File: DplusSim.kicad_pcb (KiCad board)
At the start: 2 copper layers, 40 x 60 mm, 19 parts, among them J10 K15 -, J11 Summer +, J3 Summer -, J7 Landstr. +, J8 Landstr. -, J9 K15 +, Q2 IRF7404, U5 LTV-847

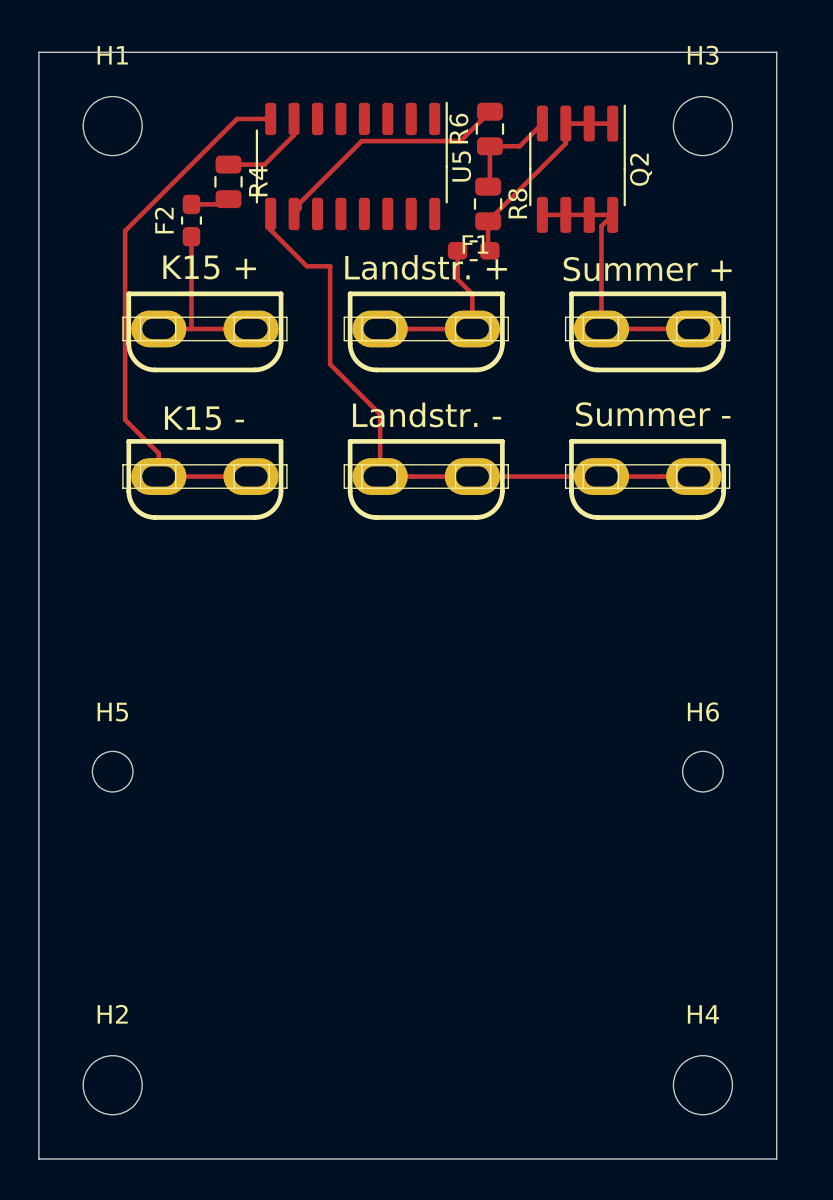
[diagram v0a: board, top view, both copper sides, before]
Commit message: x
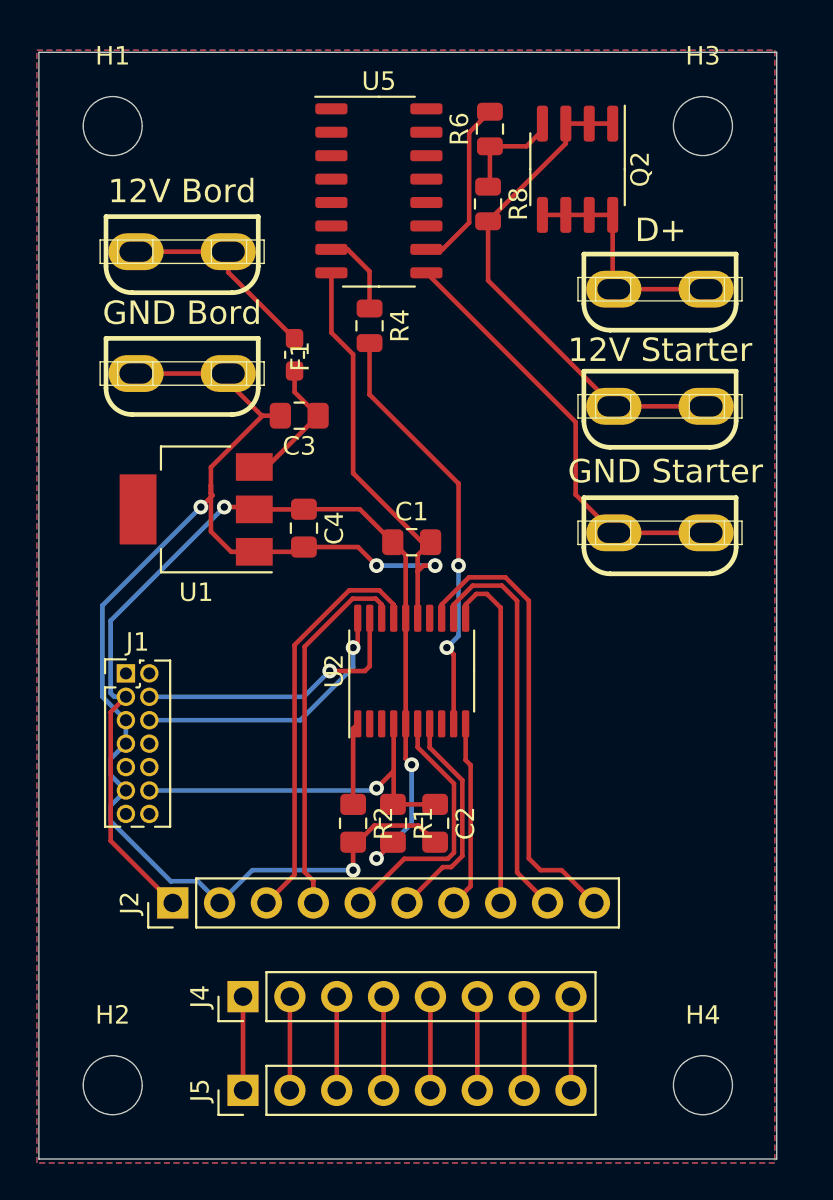
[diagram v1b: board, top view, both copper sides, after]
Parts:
- removed F2: Polyfuse, Resistor_SMD:R_0603_1608Metric_Pad1.05x0.95mm_HandSolder
- removed H5, H6: MountingHole, MountingHole:MountingHole_2.2mm_M2
- removed J10: K15 -, MyComponents:FASTON-6_3mm
- removed J9: K15 +, MyComponents:FASTON-6_3mm
- added C1: 100n, Capacitor_SMD:C_0805_2012Metric_Pad1.15x1.40mm_HandSolder, F.Cu at (29.2, 35.6)
- added C2: C, Capacitor_SMD:C_0805_2012Metric_Pad1.15x1.40mm_HandSolder, F.Cu at (30.5, 50.8)
- added C3: C, Capacitor_SMD:C_0805_2012Metric_Pad1.15x1.40mm_HandSolder, F.Cu at (23.1, 28.7)
- added C4: C, Capacitor_SMD:C_0805_2012Metric_Pad1.15x1.40mm_HandSolder, F.Cu at (23.4, 34.8)
- added J1: Conn_02x07_Odd_Even, Connector_PinHeader_1.27mm:PinHeader_2x07_P1.27mm_Vertical, F.Cu at (13.7, 42.7)
- added J2: Conn_01x10, Connector_PinHeader_2.54mm:PinHeader_1x10_P2.54mm_Vertical, F.Cu at (16.3, 55.1)
- added J4: Conn_01x08, Connector_PinHeader_2.54mm:PinHeader_1x08_P2.54mm_Vertical, F.Cu at (20.1, 60.2)
- added J5: Conn_01x08, Connector_PinHeader_2.54mm:PinHeader_1x08_P2.54mm_Vertical, F.Cu at (20.1, 65.3)
- added J6: 12V Starter, MyComponents:FASTON-6_3mm, F.Cu at (42.7, 28.2)
- added R1: R, Resistor_SMD:R_0805_2012Metric_Pad1.15x1.40mm_HandSolder, F.Cu at (28.2, 50.8)
- added R2: R, Resistor_SMD:R_0805_2012Metric_Pad1.15x1.40mm_HandSolder, F.Cu at (26.0, 50.8)
- added U1: LT1117-3.3, Package_TO_SOT_SMD:SOT-223, F.Cu at (17.5, 33.8)
- added U2: STM32L031F4Px, Package_SO:TSSOP-20_4.4x6.5mm_P0.65mm, F.Cu at (29.2, 42.5)
- J11: value Summer + -> D+
- J3: value Summer - -> GND Starter
- J7: value Landstr. + -> 12V Bord
- J8: value Landstr. - -> GND Bord
- moved J8 14.4 mm to (16.8, 26.4)
- moved J7 13.9 mm to (16.8, 19.8)
- moved F1 11.2 mm to (22.9, 25.4), turned to 90 degrees
- moved R4 10.9 mm to (26.9, 23.8)
- moved J3 3.13 mm to (42.7, 35.1)
- moved J11 2.26 mm to (42.7, 21.8)
- moved U5 1.65 mm to (27.4, 14.0), turned to 0 degrees
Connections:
- net /Warn_plus renamed /Dplus
- J3 pad 1: GND -> GNDA
- Q2 pad 1: +12V -> +12VA
- Q2 pad 2: +12V -> +12VA
- Q2 pad 3: +12V -> +12VA
- R4 pad 2: /K15_plus -> /Dplus_out
- R8 pad 2: +12V -> +12VA
- U5 pad 8: /K15_minus -> GND
- U5 pad 9: GND -> GNDA
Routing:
- net GND: track 34.4 -> 96.9 mm, vias 0 -> 4
- net +3V3: track 0.00 -> 56.0 mm, vias 0 -> 3
- net /K15_minus: track 29.5 -> 0.00 mm
- net +12VA: track 0.00 -> 27.4 mm
- net /SPI_MOSI: track 0.00 -> 25.1 mm
- net GNDA: track 0.00 -> 23.3 mm
- net /Dplus_out: track 0.00 -> 23.1 mm, vias 0 -> 2
- net /I2C_SCL: track 0.00 -> 22.3 mm
- net /SPI_MISO: track 0.00 -> 22.0 mm
- net /NRST: track 0.00 -> 20.4 mm, vias 0 -> 1
- net /I2C_SDA: track 0.00 -> 20.2 mm
- net /SPI_SCK: track 0.00 -> 19.2 mm
- net /SWDIO: track 0.00 -> 15.2 mm, vias 0 -> 1
- net /SWDCLK: track 0.00 -> 15.0 mm, vias 0 -> 1
- net /INT: track 0.00 -> 14.0 mm
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- added copper zone on B.Cu, net GND
- added copper zone on F.Cu, net GND
